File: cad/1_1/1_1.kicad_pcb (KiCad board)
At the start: 2 copper layers, 80 x 50 mm, 14 parts, among them J1 Conn_01x04_Pin, U1 ATtiny1616-M

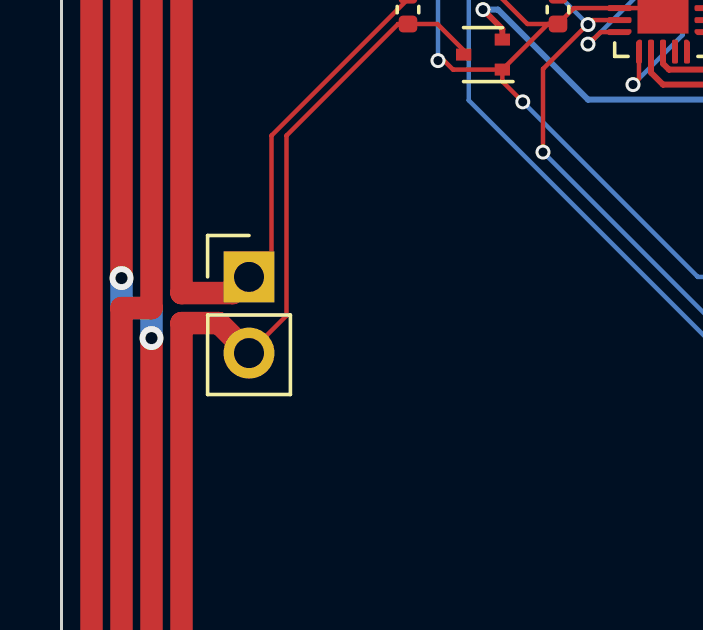
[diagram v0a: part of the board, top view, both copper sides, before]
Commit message: Update component positions and configuration in PCB design files
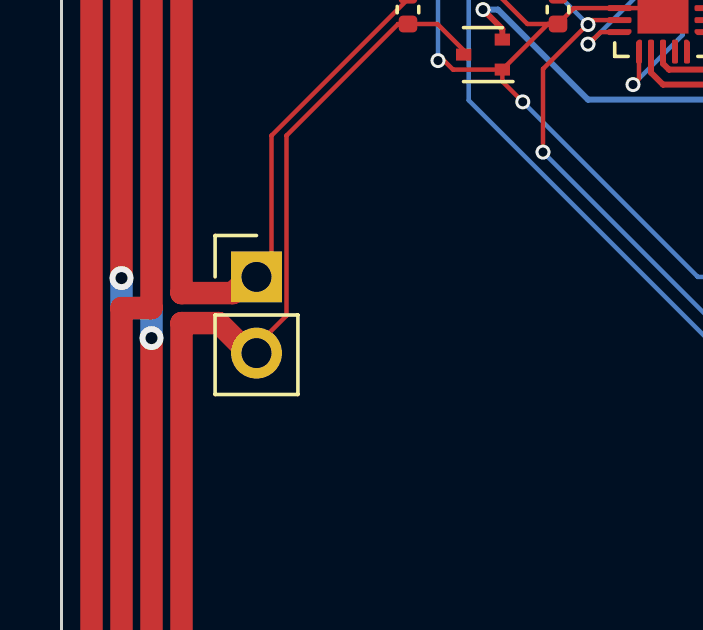
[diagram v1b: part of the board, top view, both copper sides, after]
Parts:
- moved AE1 0.25 mm to (56.5, 74.0)
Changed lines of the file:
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@@
 	(footprint "Connector_PinHeader_2.54mm:PinHeader_1x02_P2.54mm_Vertical"
 		(layer "F.Cu")
-		(at 56.25 73.96)
+		(at 56.5 73.96)
 		(descr "Through hole straight pin header, 1x02, 2.54mm pitch, single row")
 		(tags "Through hole pin header THT 1x02 2.54mm single row")
